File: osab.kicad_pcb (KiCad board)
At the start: 2 copper layers, 50 x 75 mm, 98 parts, among them CON1 TF-01A, CON2 PJ-3420-A-SMT, CON3 TYPE-C-31-M-12, Q1 BC847B, Q2 BC847B, SW1 PPP, SW10 RESET, SW11 Torch, SW2 VOL-, SW3 VOL+, SW4 CHAP-, SW5 CHAP+, SW6 OT/NT, SW7 BOOK-, SW8 BOOK+, SW9 XKB5858-Z-F, U1 VS1000, U2 ME6211C33M5G-N, U3 CAT25640, U4 TP4055, U5 MF5853CS, U6 PAM8302AAS, Y1 12MHz

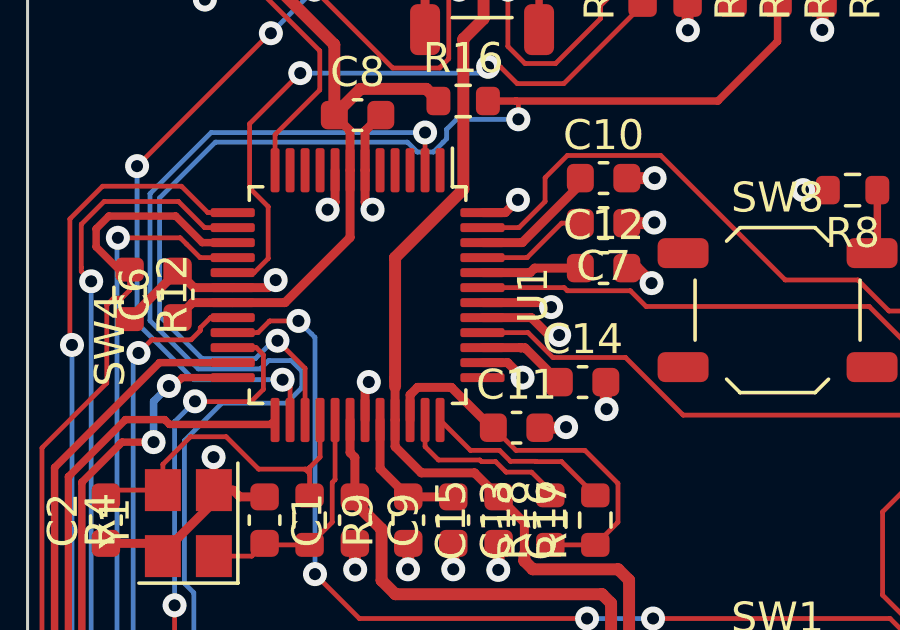
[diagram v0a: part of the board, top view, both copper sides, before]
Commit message: production: Routing tracks...
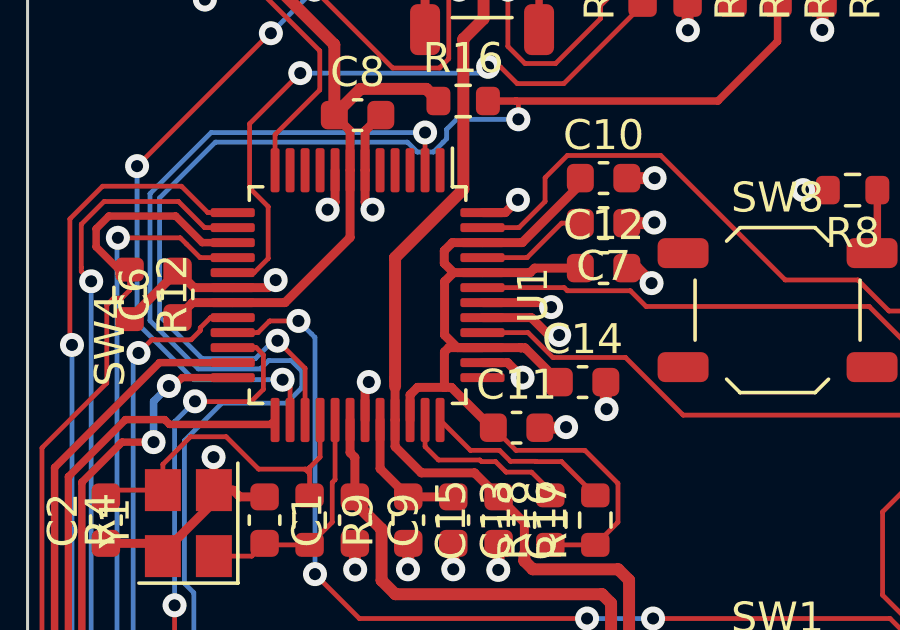
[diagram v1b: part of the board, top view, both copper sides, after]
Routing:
- net AVDD: track 24.6 -> 33.9 mm
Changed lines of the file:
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@@
   (segment (start 143.175 80.55) (end 143.425 80.8) (width 0.3) (layer "F.Cu") (net 9))
   (segment (start 141.27952 88.17452) (end 143.577663 88.17452) (width 0.16) (layer "F.Cu") (net 10))
+  (segment (start 139.16 81.25) (end 138.89 81.52) (width 0.3) (layer "F.Cu") (net 10))
+  (segment (start 138.9 82.55) (end 139.2 82.25) (width 0.3) (layer "F.Cu") (net 10))
   (segment (start 141.75 82.25) (end 141.9 82.1) (width 0.3) (layer "F.Cu") (net 10))
   (segment (start 144.67952 90.57048) (end 143.925 91.325) (width 0.16) (layer "F.Cu") (net 10))
+  (segment (start 138.89548 86.07548) (end 139.12548 86.07548) (width 0.3) (layer "F.Cu") (net 10))
   (segment (start 137.75 87.1625) (end 137.75 86.324639) (width 0.3) (layer "F.Cu") (net 10))
   (segment (start 141.43516 84.75) (end 141.444182 84.759022) (width 0.3) (layer "F.Cu") (net 10))
@@
   (segment (start 143.425 79.312507) (end 143.425 79.1) (width 0.3) (layer "F.Cu") (net 10))
   (segment (start 141.487507 81.25) (end 143.425 79.312507) (width 0.3) (layer "F.Cu") (net 10))
+  (segment (start 138.89 81.52) (end 138.89 81.94) (width 0.3) (layer "F.Cu") (net 10))
+  (segment (start 139.32 84.75) (end 138.9 84.33) (width 0.3) (layer "F.Cu") (net 10))
+  (segment (start 140.1625 84.75) (end 139.32 84.75) (width 0.3) (layer "F.Cu") (net 10))
+  (segment (start 140.1625 81.25) (end 139.16 81.25) (width 0.3) (layer "F.Cu") (net 10))
   (segment (start 143.362507 79.3) (end 143.45 79.3) (width 0.3) (layer "F.Cu") (net 10))
+  (segment (start 138.89548 84.89452) (end 139.04 84.75) (width 0.3) (layer "F.Cu") (net 10))
   (segment (start 140.1625 84.75) (end 141.43516 84.75) (width 0.3) (layer "F.Cu") (net 10))
   (segment (start 140.1625 81.25) (end 141.487507 81.25) (width 0.3) (layer "F.Cu") (net 10))
+  (segment (start 139.04 84.75) (end 140.1625 84.75) (width 0.3) (layer "F.Cu") (net 10))
   (segment (start 140.47 87.42) (end 140.525 87.42) (width 0.3) (layer "F.Cu") (net 10))
+  (segment (start 137.999159 86.07548) (end 138.89548 86.07548) (width 0.3) (layer "F.Cu") (net 10))
+  (segment (start 138.9 84.33) (end 138.9 82.55) (width 0.3) (layer "F.Cu") (net 10))
   (segment (start 141.9 82.1) (end 143.425 82.1) (width 0.3) (layer "F.Cu") (net 10))
-  (segment (start 137.999159 86.07548) (end 139.12548 86.07548) (width 0.3) (layer "F.Cu") (net 10))
   (segment (start 142.425 91.325) (end 144.2 91.325) (width 0.16) (layer "F.Cu") (net 10))
   (segment (start 141.444182 84.759022) (end 141.584022 84.759022) (width 0.3) (layer "F.Cu") (net 10))
+  (segment (start 138.89 81.94) (end 139.2 82.25) (width 0.3) (layer "F.Cu") (net 10))
   (segment (start 139.12548 86.07548) (end 140.47 87.42) (width 0.3) (layer "F.Cu") (net 10))
   (segment (start 140.1625 82.25) (end 141.75 82.25) (width 0.3) (layer "F.Cu") (net 10))
@@
   (segment (start 141.584022 84.759022) (end 142.725 85.9) (width 0.3) (layer "F.Cu") (net 10))
   (segment (start 140.525 87.42) (end 141.27952 88.17452) (width 0.16) (layer "F.Cu") (net 10))
+  (segment (start 138.89548 86.07548) (end 138.89548 84.89452) (width 0.3) (layer "F.Cu") (net 10))
+  (segment (start 139.2 82.25) (end 140.1625 82.25) (width 0.3) (layer "F.Cu") (net 10))
   (segment (start 143.425 82.087493) (end 143.425 82.4) (width 0.3) (layer "F.Cu") (net 10))
   (segment (start 152.19 115.69) (end 155.03 115.69) (width 0.25) (layer "F.Cu") (net 11))

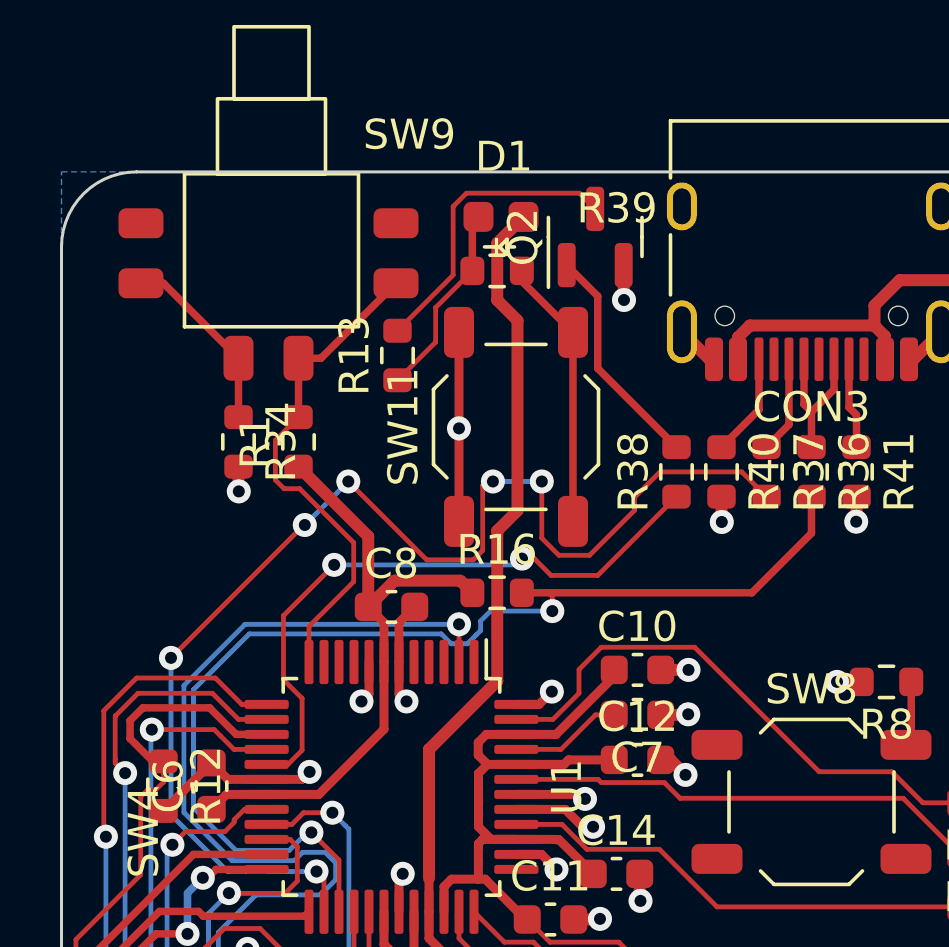
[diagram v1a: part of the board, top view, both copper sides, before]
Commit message: production: Routing tracks...
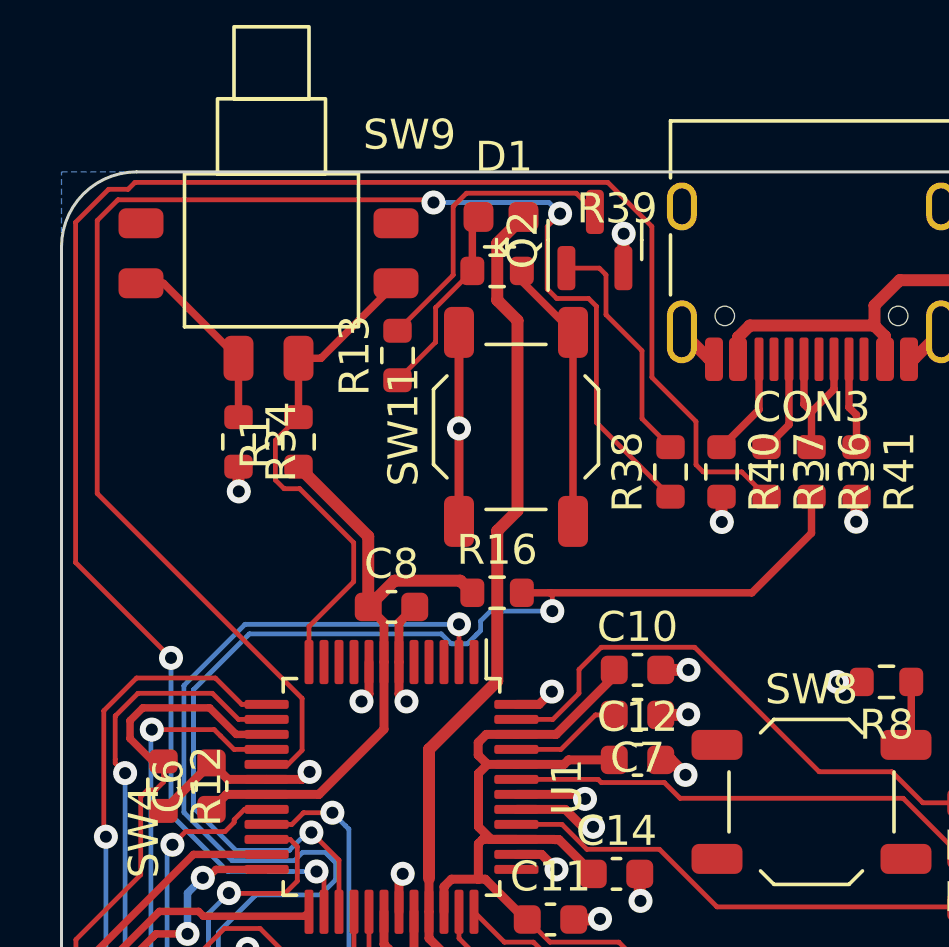
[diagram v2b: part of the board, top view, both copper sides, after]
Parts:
- moved R38 0.20 mm to (145.3, 72.5)
- moved Q2 0.10 mm to (142.8, 64.8)
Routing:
- net Net-(R38-Pad1): track 21.3 -> 49.7 mm
- net Net-(R37-Pad2): track 41.9 -> 59.9 mm, vias 6 -> 2
